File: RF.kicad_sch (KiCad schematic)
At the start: 18 parts, among them J1 USB_C_Receptacle_USB2.0_16P, J3 SMA PCB END LAUNCH JACK ROUND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, U3 USBLC6-2SC6

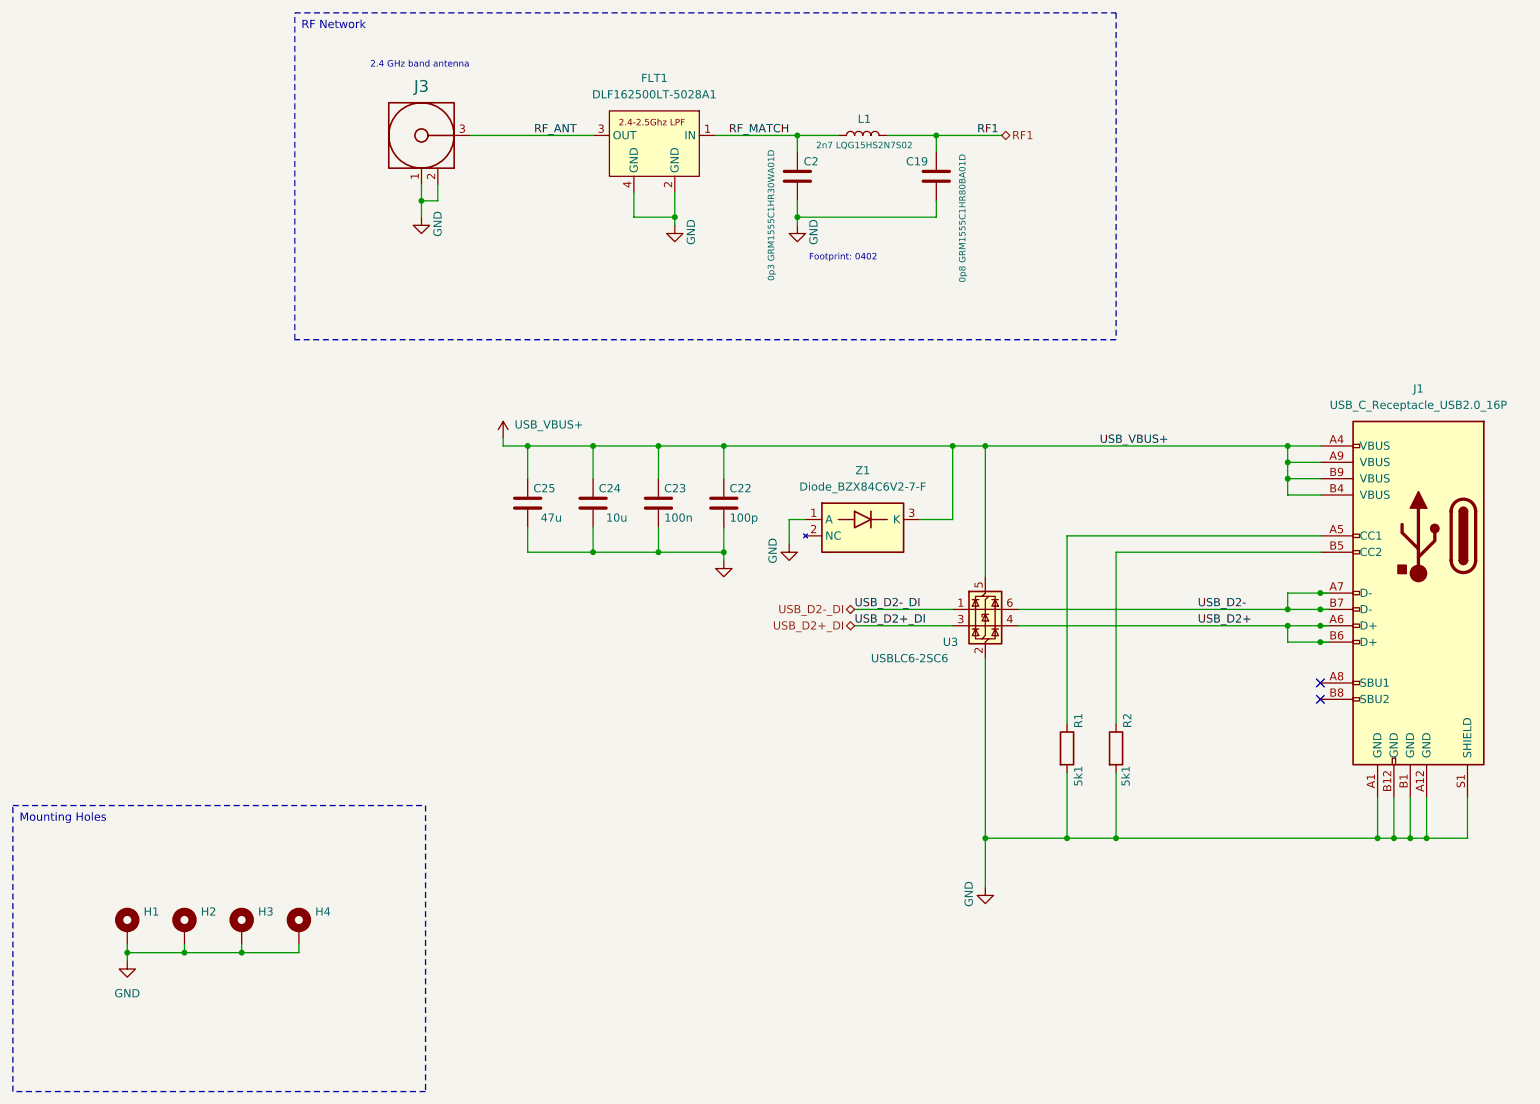
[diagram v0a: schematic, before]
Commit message: Update
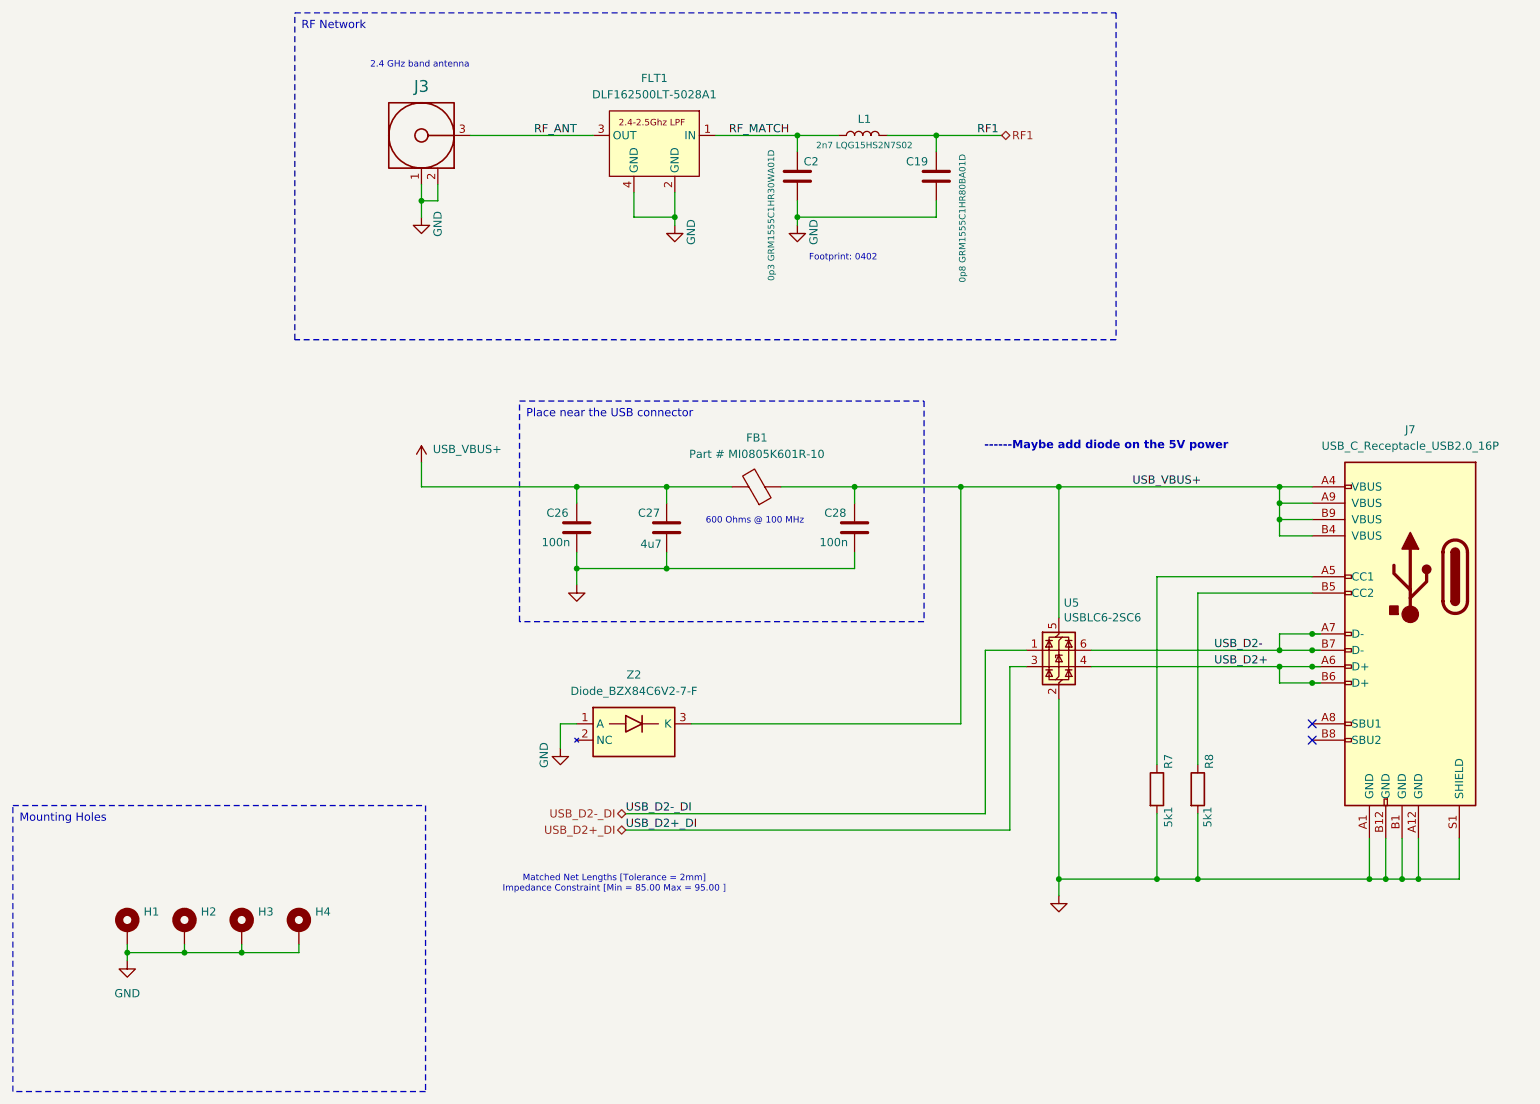
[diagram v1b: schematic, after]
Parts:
- removed C22: 100p, Capacitor_SMD:C_0805_2012Metric, symbol Device:C
- removed C23: 100n, Capacitor_SMD:C_0805_2012Metric, symbol Device:C
- removed C24: 10u, Capacitor_SMD:C_0805_2012Metric, symbol Device:C
- removed C25: 47u, Capacitor_SMD:C_0805_2012Metric, symbol Device:C
- removed J1: USB_C_Receptacle_USB2.0_16P, Connector_USB:USB_C_Receptacle_HRO_TYPE-C-31-M-12, symbol Connector:USB_C_Receptacle_USB2.0_16P
- removed R1, R2: 5k1, Resistor_SMD:R_0805_2012Metric, symbol Device:R
- removed U3: USBLC6-2SC6, Package_TO_SOT_SMD:SOT-23-6, symbol Power_Protection:USBLC6-2SC6
- removed Z1: Diode_BZX84C6V2-7-F, Personal_Project:Diode_BZX84C6V2_SOT96P240X110-3N, symbol Personal_Projects:Diode_BZX84C6V2-7-F
- added C26, C28: 100n, Capacitor_SMD:C_0805_2012Metric, symbol Device:C
- added C27: 4u7, Capacitor_SMD:C_0805_2012Metric, symbol Device:C
- added FB1: Part # MI0805K601R-10, Capacitor_SMD:C_0805_2012Metric, symbol Device:FerriteBead
- added J7: USB_C_Receptacle_USB2.0_16P, Connector_USB:USB_C_Receptacle_HRO_TYPE-C-31-M-12, symbol Connector:USB_C_Receptacle_USB2.0_16P
- added R7, R8: 5k1, Resistor_SMD:R_0805_2012Metric, symbol Device:R
- added U5: USBLC6-2SC6, Package_TO_SOT_SMD:SOT-23-6, symbol Power_Protection:USBLC6-2SC6
- added Z2: Diode_BZX84C6V2-7-F, Personal_Project:Diode_BZX84C6V2_SOT96P240X110-3N, symbol Personal_Projects:Diode_BZX84C6V2-7-F
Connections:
- net GND: now also C26.2, C27.2, C28.2, J7.A1 (GND), J7.A12 (GND), J7.B1 (GND), J7.B12 (GND), J7.S1 (SHIELD), R7.2, R8.2, U5.2 (GND), Z2.1 (A)
- net USB_D2+: now also J7.A6 (D+), J7.B6 (D+), U5.4 (I/O2)
- net USB_D2+_DI: now also U5.3 (I/O2)
- net USB_D2-: now also J7.A7 (D-), J7.B7 (D-), U5.6 (I/O1)
- net USB_D2-_DI: now also U5.1 (I/O1)
- net USB_VBUS+: now also C26.1, C27.1, C28.1, FB1.1, FB1.2, J7.A4 (VBUS), J7.A9 (VBUS), J7.B4 (VBUS), J7.B9 (VBUS), U5.5 (VBUS), Z2.3 (K)
- new net: J7.A5 (CC1), R7.1
- new net: J7.B5 (CC2), R8.1
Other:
- note added: "------Maybe add diode on the 5V power"
- note added: "600 Ohms @ 100 MHz"
- note added: "Matched Net Lengths [Tolerance = 2mm] Impedance Constraint [Min = 85.00 Max = 95.00 ]"
